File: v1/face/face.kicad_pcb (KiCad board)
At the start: 2 copper layers, 84 x 84 mm, 0 parts

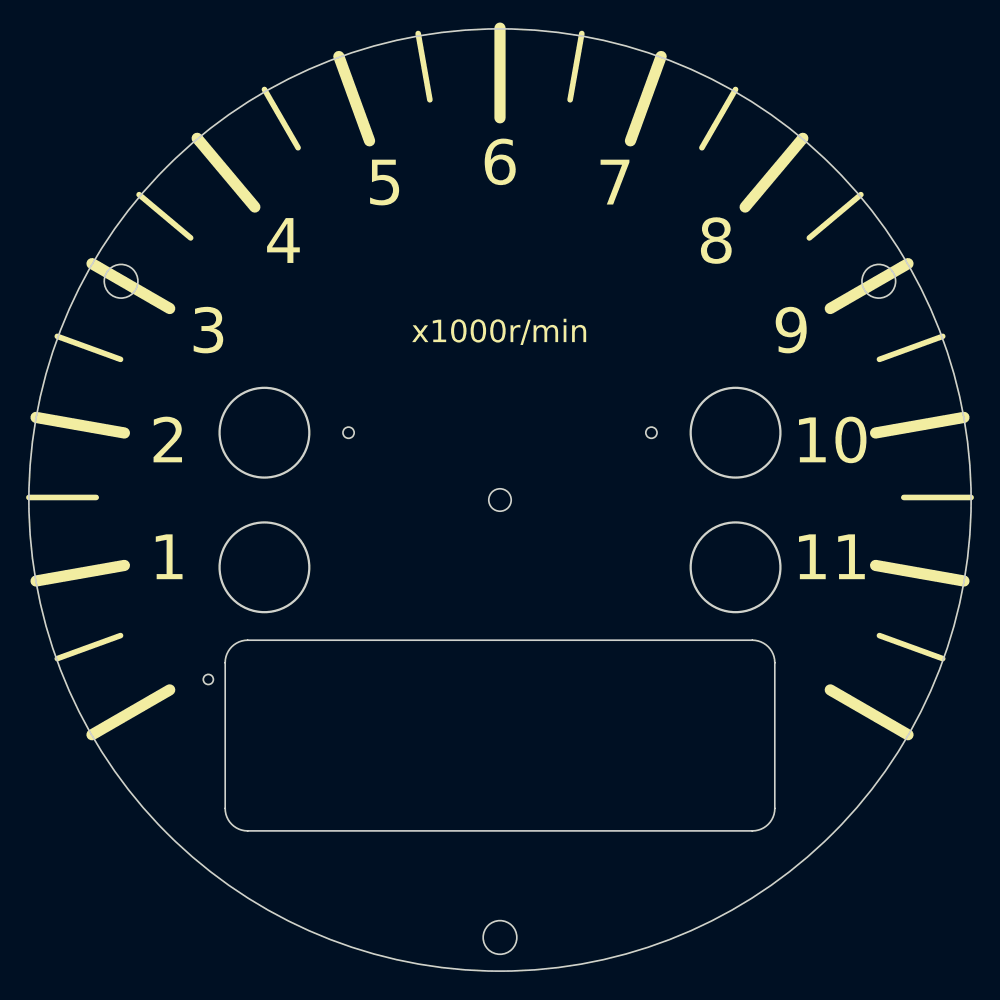
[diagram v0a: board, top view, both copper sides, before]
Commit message: Stuff
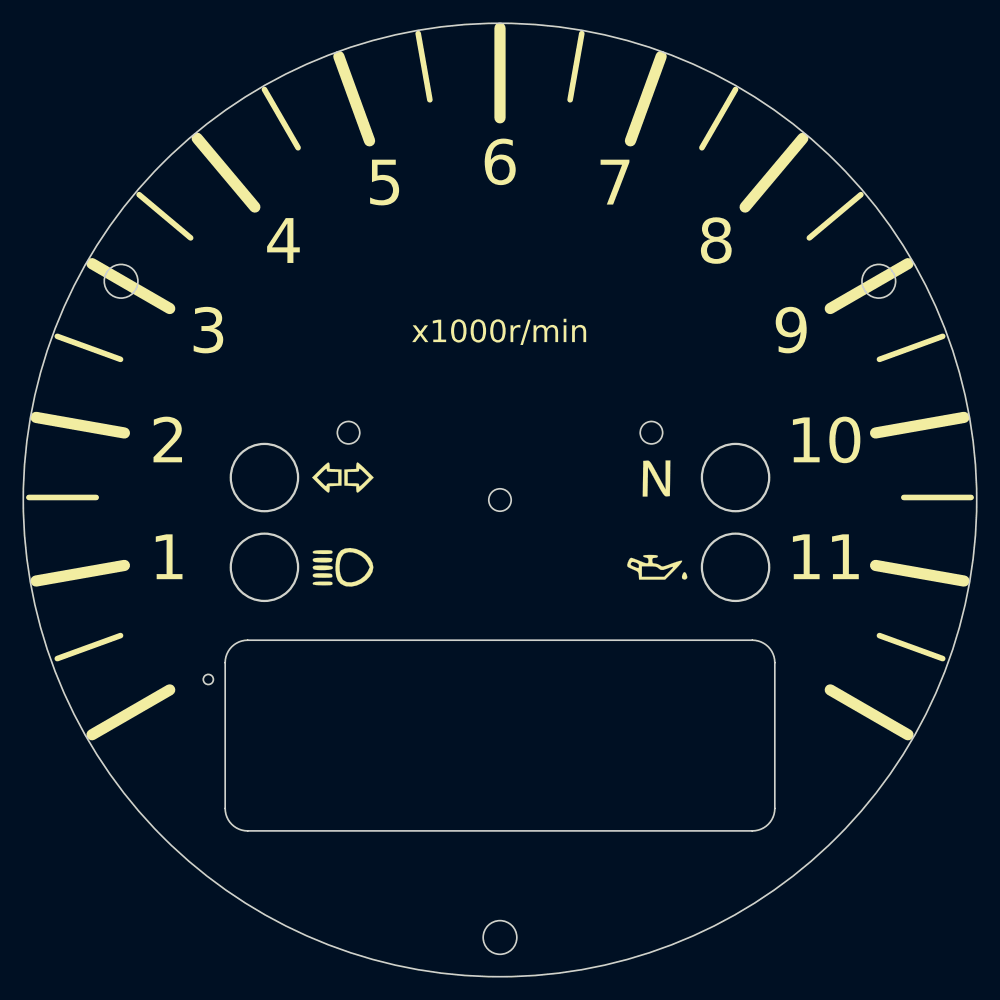
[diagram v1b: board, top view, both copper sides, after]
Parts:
- added G***: LOGO, footprints:high-beam, F.Cu at (136.0, 106.0)
- added G***: LOGO, footprints:turn-signals, F.Cu at (136.0, 98.0)
- added G***: LOGO, footprints:neutral, F.Cu at (164.0, 98.0)
- added G***: LOGO, footprints:oil, F.Cu at (164.0, 106.0)
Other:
- board size 84 x 84 mm -> 85 x 85 mm

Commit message: Stuff
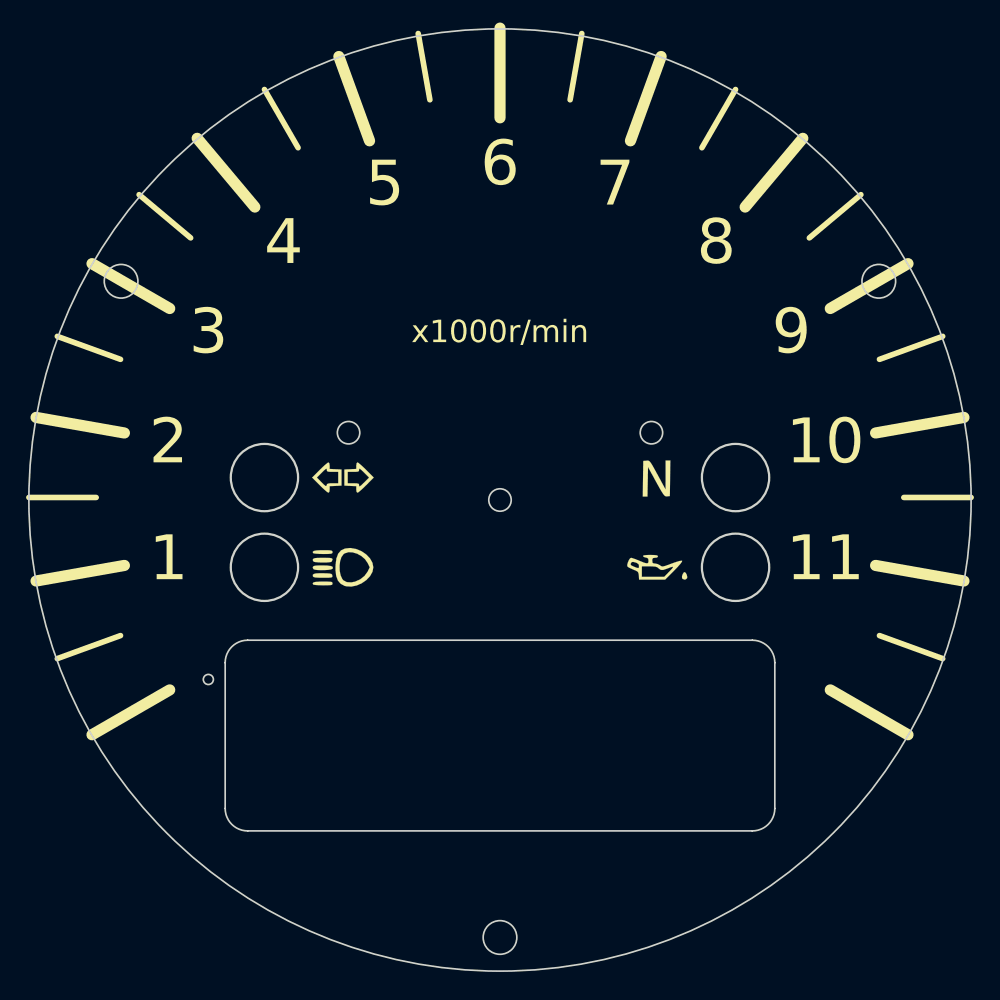
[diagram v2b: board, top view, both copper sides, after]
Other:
- board size 85 x 85 mm -> 84 x 84 mm
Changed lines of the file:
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@@
       (drillshape 0)
       (scaleselection 1)
-      (outputdirectory "face_gerber"))
+      (outputdirectory "gerber"))
   )
   (net 0 "")
@@
     (effects (font (size 4 4) (thickness 0.3)))
   )
-  (gr_circle (center 150 100) (end 192.5 100) (layer Edge.Cuts) (width 0.15))
+  (gr_circle (center 150 100) (end 192 100) (layer Edge.Cuts) (width 0.15))
 )
